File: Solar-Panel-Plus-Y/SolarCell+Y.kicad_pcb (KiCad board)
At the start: 6 copper layers, 50 x 50 mm, 75 parts, among them J1 symbols_XF2M-1015-1A, J2 U.FL-R-SMT-1, Q1 IRLML2803, U1 TTB12G51-Balun, U2 NDS8434, U3 TSL2561, U4 Value

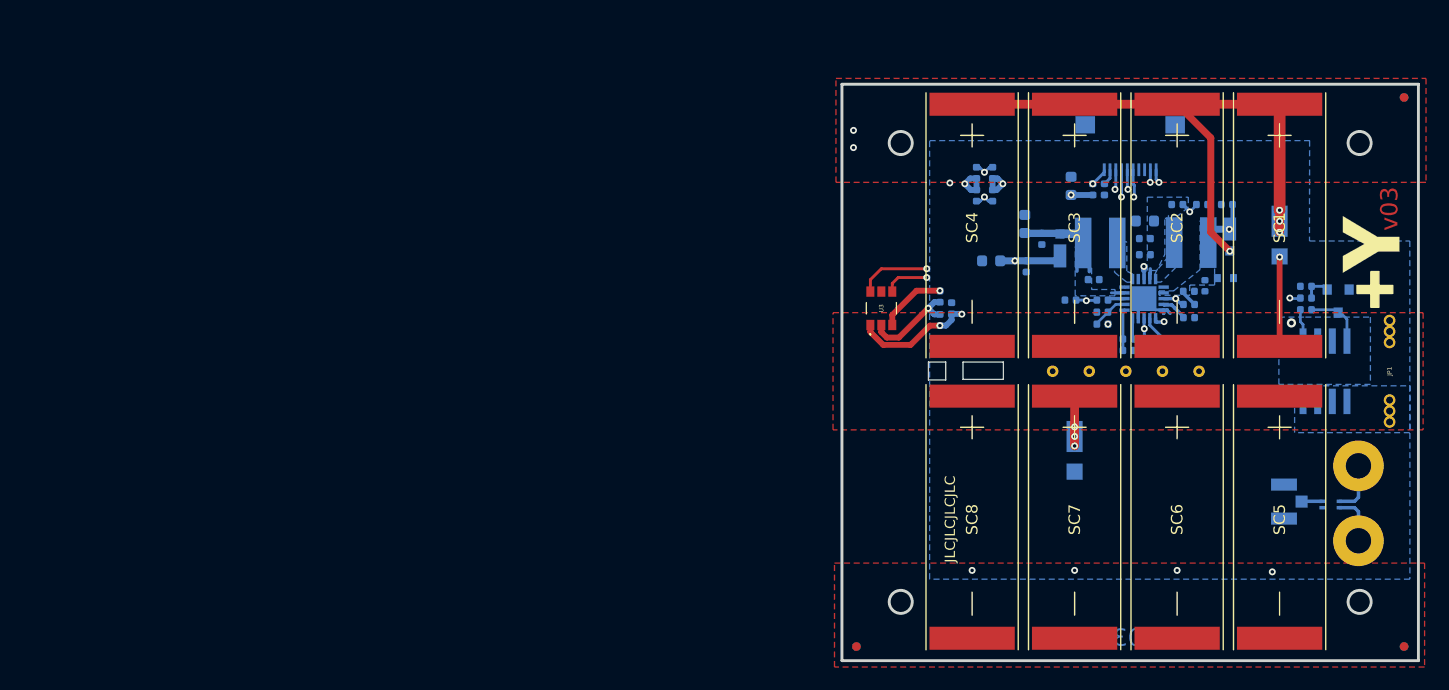
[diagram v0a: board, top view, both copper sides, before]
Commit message: Made Requested Changes
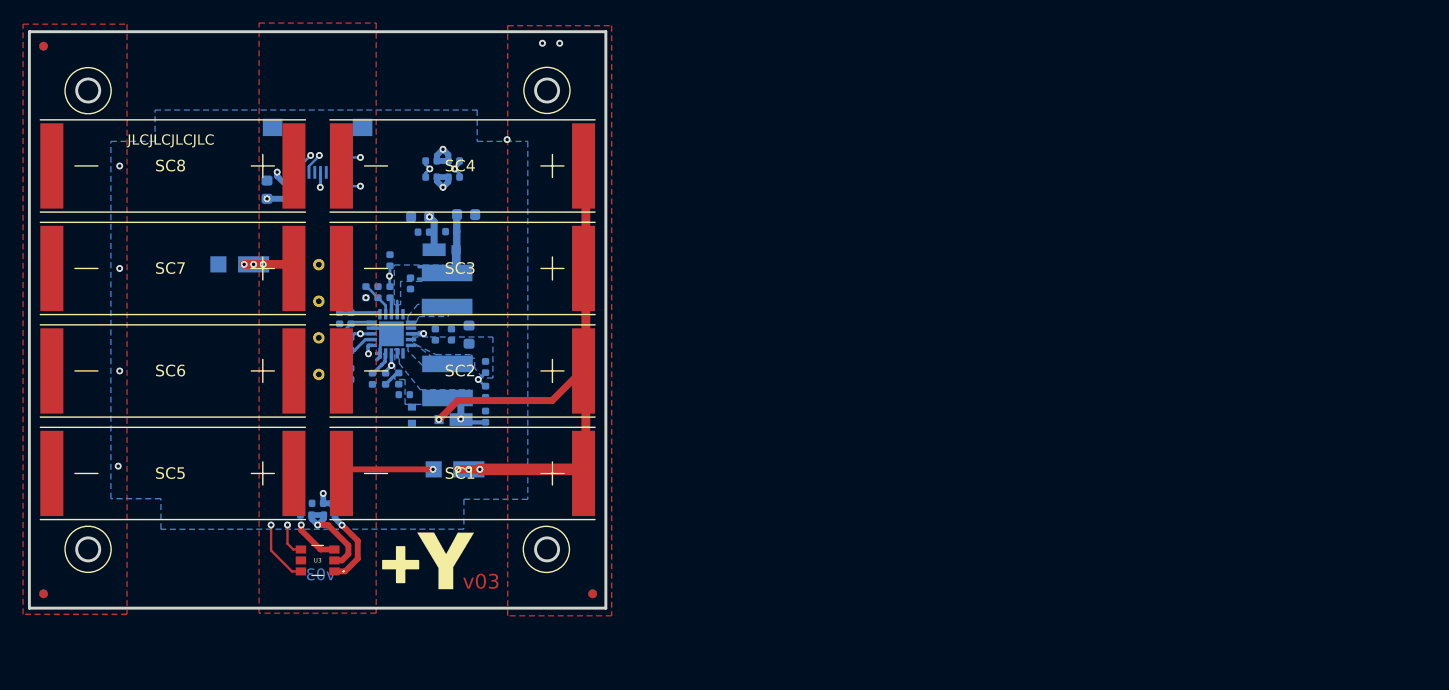
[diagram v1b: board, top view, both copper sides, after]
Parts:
- removed H1, H2: MountingHole_Pad, MountingHole:MountingHole_2.2mm_M2_Pad
- removed J2: U.FL-R-SMT-1, misc-circuits:U.FL-R-SMT-1
- removed JP1: Jumper, SolarCellParts:Burn Wire
- removed Q1: IRLML2803, Package_TO_SOT_SMD:SOT-23
- removed R5, R7: 1M, Resistor_SMD:R_0402_1005Metric
- removed R6: 4.7k, Resistor_SMD:R_0402_1005Metric
- removed TP5: TP, TestPoint:TestPoint_THTPad_D1.0mm_Drill0.5mm
- removed U1: TTB12G51-Balun, misc-circuits:TTB12G51-balun
- removed U2: NDS8434, misc-circuits:NDS8434
- moved REF** 118.1 mm to (80.8, 84.2), turned to -90 degrees (x2)
- moved REF** 87.6 mm to (80.8, 36.7), turned to -90 degrees (x2)
- moved SC5 85.8 mm to (102.5, 73.8), turned to 180 degrees
- moved REF** 82.5 mm to (128.4, 84.2), turned to -90 degrees (x2)
- moved Ref** 78.6 mm to (132.7, 82.3), turned to 0 degrees
- moved SC6 76.6 mm to (102.5, 64.9), turned to 180 degrees
- moved D1 74.4 mm to (116.4, 73.4), turned to 180 degrees
- moved D2 74.2 mm to (97.8, 55.6), turned to 180 degrees
- moved TP4 73.2 mm to (104.6, 65.2), turned to -90 degrees
- moved R16 72.3 mm to (107.4, 65.1), turned to 90 degrees
- moved D5 71.6 mm to (112.7, 68.7), turned to -90 degrees
- moved C4 71.0 mm to (109.3, 65.5), turned to -90 degrees
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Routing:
- net /coil: track 13156.8 -> 12938.3 mm
- net BURN1: track 31.3 -> 0.00 mm, vias 2 -> 0
- net BATT_P: track 38.3 -> 22.1 mm, vias 2 -> 1
- net SDA1: track 27.2 -> 40.8 mm
- net SCL1: track 26.1 -> 38.3 mm
- net /VBAT: track 13.7 -> 24.8 mm
- net COIL_P: track 22.4 -> 13.4 mm
- net Net-(Q1-Pad3): track 5.31 -> 0.00 mm
- net Net-(H2-Pad1): track 4.52 -> 0.00 mm
- net Net-(H1-Pad1): track 4.32 -> 0.00 mm
- net COIL_N: track 17.5 -> 13.3 mm
- net Net-(Q1-Pad1): track 2.49 -> 0.00 mm
- net VSOLAR: track 22.6 -> 20.4 mm
- net GND: track 9.03 -> 7.13 mm
- net Net-(J2-Pad3): track 1.80 -> 0.00 mm
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- removed copper zone on B.Cu, net /VBURN
- removed copper zone on B.Cu, net BATT_P
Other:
- outline, holes or cut-outs redrawn
- rule pad_to_mask_clearance: 0.049 -> 0.0508
- board text removed: "BURN"
